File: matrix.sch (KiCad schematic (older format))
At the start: 143 parts

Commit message: Update: Work on PCB component placement
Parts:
- K_,1, K_.1, K_/1, K_;1, K_A1, K_B1, K_C1, K_D1, K_E1, K_F1, K_FN3, K_FN4_2, K_G1, K_H1, K_I1, K_J1, K_K1, K_L1, K_LALT1, K_M1, K_N1, K_O1, K_P1, K_Q1, K_R1, K_S1, K_T1, K_TAB1, K_U1, K_V1, K_W1, K_X1, K_Y1, K_Z1: footprint MX_Alps_Hybrid:MX-1U -> MX_Alps_Hybrid:MXOnly-1U
- K_BACK1, K_LSHIFT1: footprint MX_Alps_Hybrid:MX-1.75U -> MX_Alps_Hybrid:MXOnly-1.75U
- K_FN1: footprint MX_Alps_Hybrid:MX-1.25U -> MX_Alps_Hybrid:MXOnly-1.25U
- K_FN2: footprint MX_Alps_Hybrid:MX-1.5U -> MX_Alps_Hybrid:MXOnly-1.5U
- K_LCTL2, K_SUPER2: footprint MX_Alps_Hybrid:MX-1U -> MX_Alps_Hybrid:MXOnly-1U-FLIPPED

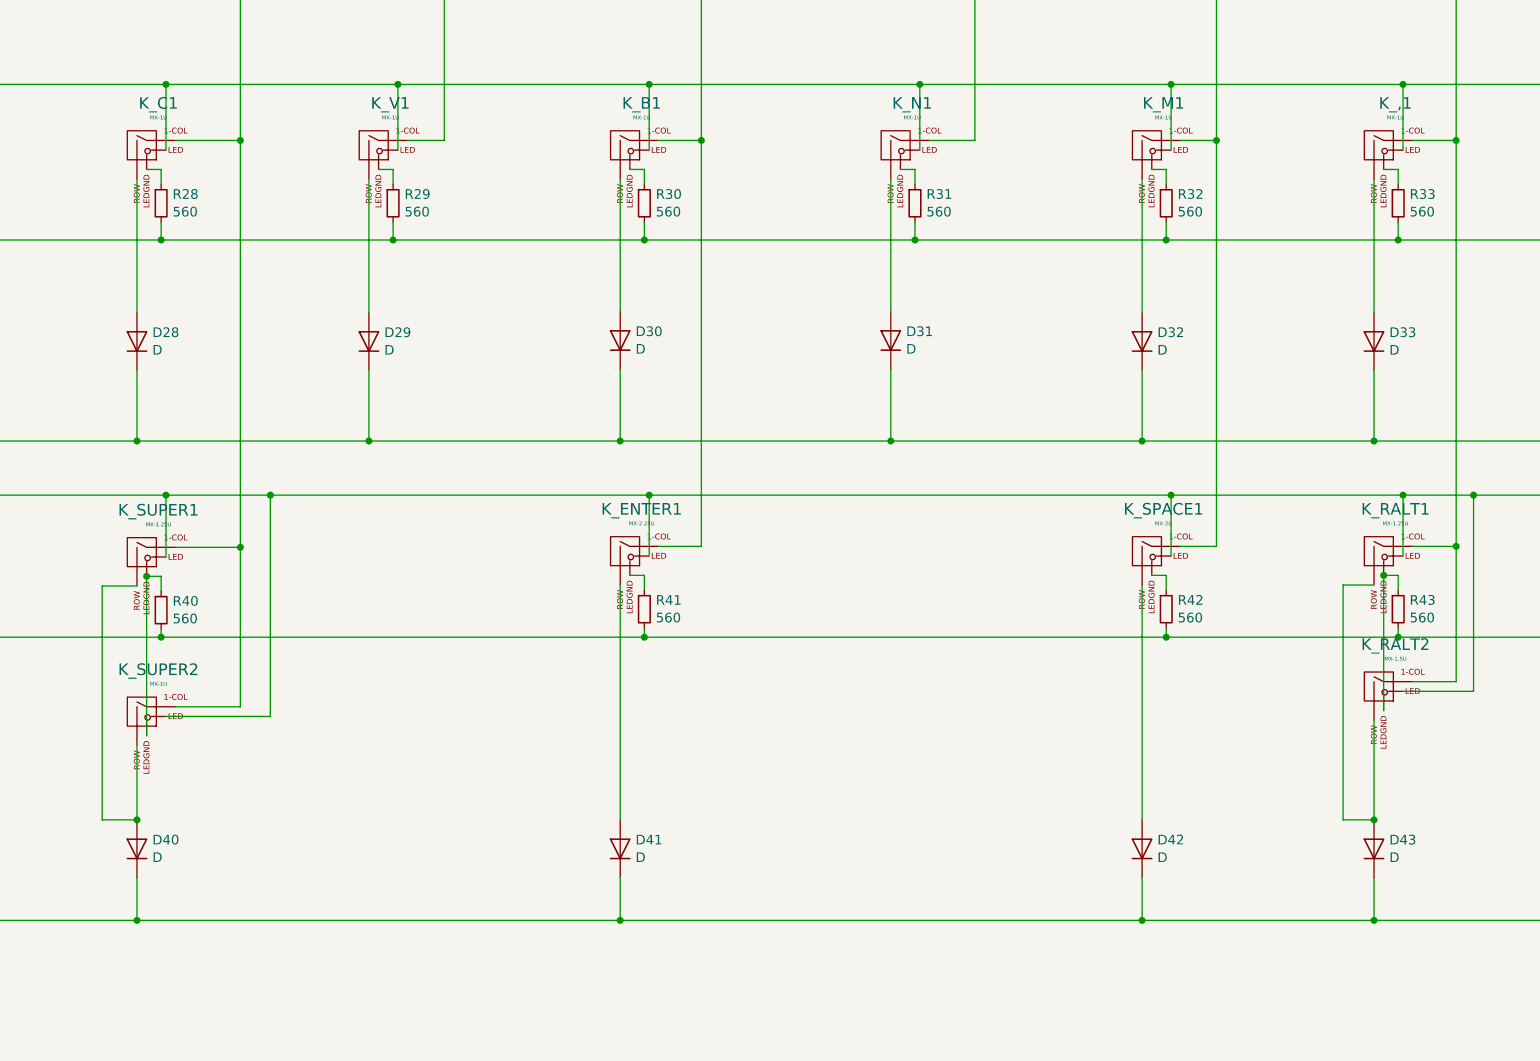
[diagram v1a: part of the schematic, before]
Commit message: Update: Work on PCB layout
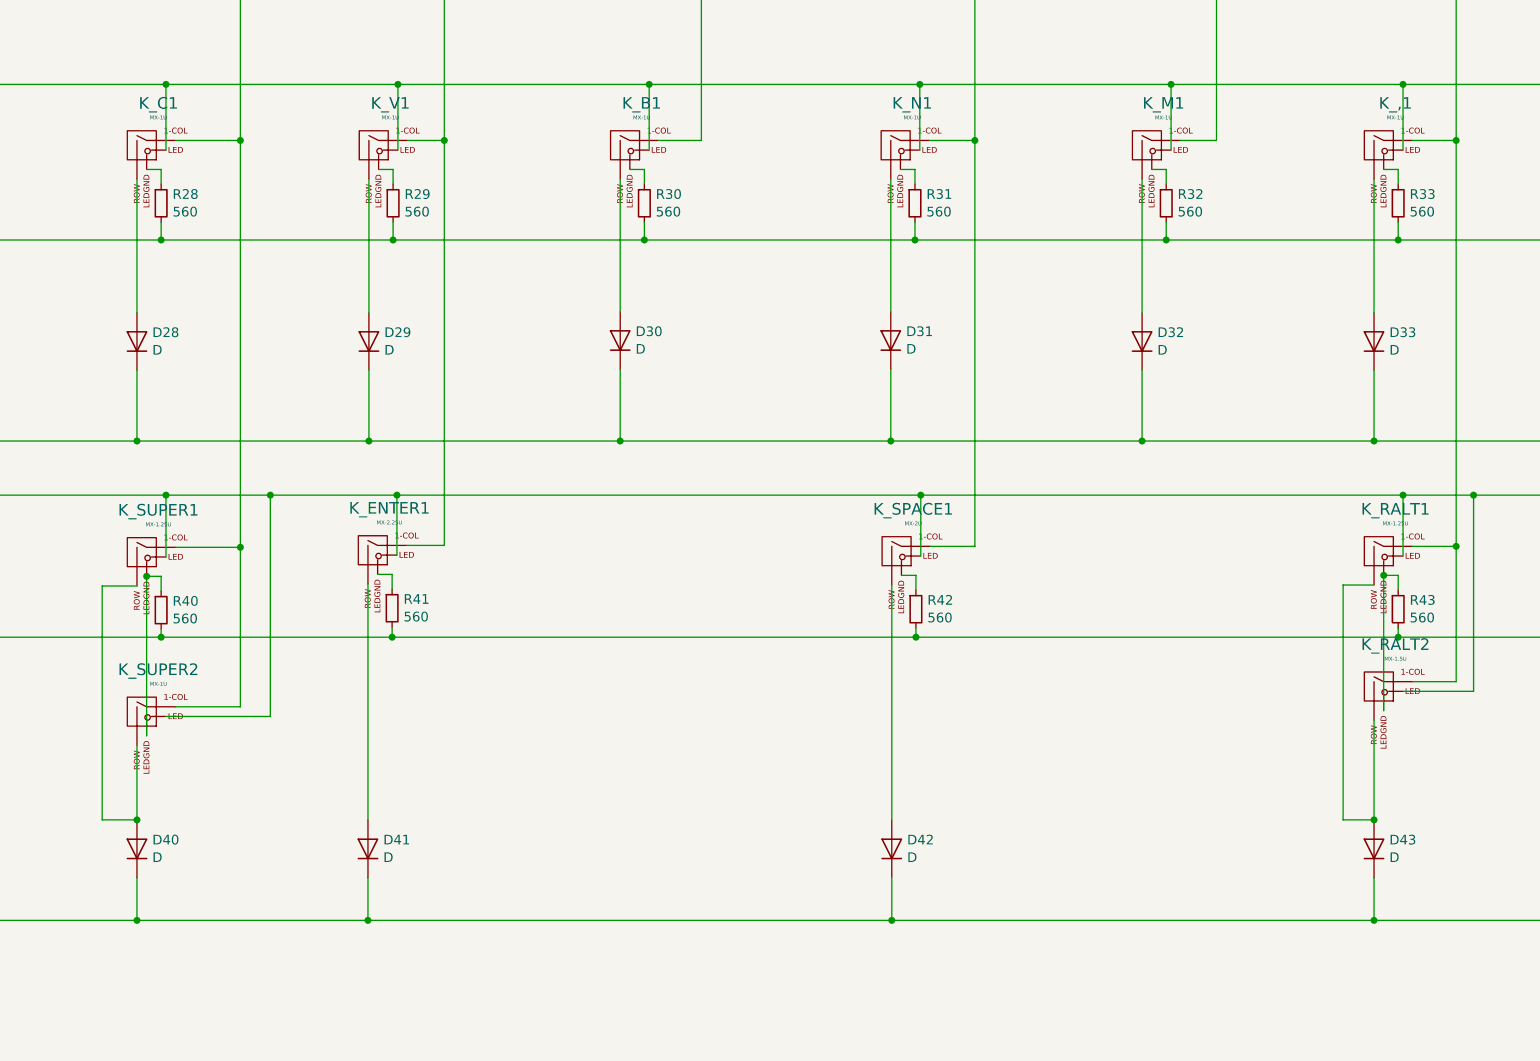
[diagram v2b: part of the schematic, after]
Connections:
- net COL4: now also K_ENTER1.1 (COL)
- net COL5: no longer K_ENTER1.1 (COL)
- net COL6: now also K_SPACE1.1 (COL)
- net COL7: no longer K_SPACE1.1 (COL)
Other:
- moved on the sheet: D41, D42, K_ENTER1, K_SPACE1, R41, R42
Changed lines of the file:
@@
 L MX_Alps_Hybrids:MX-2.25U K_ENTER1
 U 1 1 5C22137B
-P 7200 6800
-F 0 "K_ENTER1" H 7286 7017 60  0000 C CNN
-F 1 "MX-2.25U" H 7286 6943 20  0000 C CNN
-F 2 "MX_Alps_Hybrid:MXOnly-2.25U-ReversedStabilizers" H 7175 6775 60  0001 C CNN
-F 3 "" H 7175 6775 60  0001 C CNN
-	1    7200 6800
+P 5895 6795
+F 0 "K_ENTER1" H 5981 7012 60  0000 C CNN
+F 1 "MX-2.25U" H 5981 6938 20  0000 C CNN
+F 2 "MX_Alps_Hybrid:MXOnly-2.25U-ReversedStabilizers" H 5870 6770 60  0001 C CNN
+F 3 "" H 5870 6770 60  0001 C CNN
+	1    5895 6795
 	1    0    0    -1
 $EndComp
@@
 L MX_Alps_Hybrids:MX-2U K_SPACE1
 U 1 1 5C223C71
-P 9900 6800
-F 0 "K_SPACE1" H 9986 7017 60  0000 C CNN
-F 1 "MX-2U" H 9986 6943 20  0000 C CNN
-F 2 "MX_Alps_Hybrid:MXOnly-2U-ReversedStabilizers" H 9875 6775 60  0001 C CNN
-F 3 "" H 9875 6775 60  0001 C CNN
-	1    9900 6800
+P 8605 6800
+F 0 "K_SPACE1" H 8691 7017 60  0000 C CNN
+F 1 "MX-2U" H 8691 6943 20  0000 C CNN
+F 2 "MX_Alps_Hybrid:MXOnly-2U-ReversedStabilizers" H 8580 6775 60  0001 C CNN
+F 3 "" H 8580 6775 60  0001 C CNN
+	1    8605 6800
 	1    0    0    -1
 $EndComp
@@
 L Device:R_Small R41
 U 1 1 5C24348B
-P 7300 7100
-F 0 "R41" H 7359 7146 50  0000 L CNN
-F 1 "560" H 7359 7055 50  0000 L CNN
-F 2 "Resistor_SMD:R_0603_1608Metric" H 7300 7100 50  0001 C CNN
-F 3 "~" H 7300 7100 50  0001 C CNN
-	1    7300 7100
+P 5995 7095
+F 0 "R41" H 6054 7141 50  0000 L CNN
+F 1 "560" H 6054 7050 50  0000 L CNN
+F 2 "Resistor_SMD:R_0603_1608Metric" H 5995 7095 50  0001 C CNN
+F 3 "~" H 5995 7095 50  0001 C CNN
+	1    5995 7095
 	1    0    0    -1
 $EndComp
@@
 L Device:R_Small R42
 U 1 1 5C2440AF
-P 10000 7100
-F 0 "R42" H 10059 7146 50  0000 L CNN
-F 1 "560" H 10059 7055 50  0000 L CNN
-F 2 "Resistor_SMD:R_0603_1608Metric" H 10000 7100 50  0001 C CNN
-F 3 "~" H 10000 7100 50  0001 C CNN
-	1    10000 7100
+P 8705 7100
+F 0 "R42" H 8764 7146 50  0000 L CNN
+F 1 "560" H 8764 7055 50  0000 L CNN
+F 2 "Resistor_SMD:R_0603_1608Metric" H 8705 7100 50  0001 C CNN
+F 3 "~" H 8705 7100 50  0001 C CNN
+	1    8705 7100
 	1    0    0    -1
 $EndComp
@@
 	4800 6930 4800 7005
 Wire Wire Line
-	7225 6925 7300 6925
-Wire Wire Line
-	7300 6925 7300 7000
-Wire Wire Line
-	9925 6925 10000 6925
-Wire Wire Line
-	10000 6925 10000 7000
+	5920 6920 5995 6920
+Wire Wire Line
+	5995 6920 5995 6995
+Wire Wire Line
+	8630 6925 8705 6925
+Wire Wire Line
+	8705 6925 8705 7000
 Wire Wire Line
 	11125 6925 11200 6925
@@
 Connection ~ 2300 7245
 Wire Wire Line
-	7300 7200 7300 7245
-Wire Wire Line
-	10000 7200 10000 7245
-Wire Wire Line
-	10000 7245 7300 7245
-Connection ~ 7300 7245
-Wire Wire Line
 	11200 7200 11200 7245
-Wire Wire Line
-	11200 7245 10000 7245
-Connection ~ 10000 7245
 Wire Wire Line
 	12500 7200 12500 7245
@@
 	11225 6510 11225 6825
 Connection ~ 12525 6510
-Wire Wire Line
-	10025 6510 10025 6825
 Connection ~ 11225 6510
-Wire Wire Line
-	7325 6510 7325 6825
-Connection ~ 10025 6510
-Connection ~ 7325 6510
 Wire Wire Line
 	2325 6510 2325 6825
@@
 COL5
 Wire Wire Line
-	7375 6775 7595 6775
-Wire Wire Line
 	7595 750  7595 1275
 Wire Wire Line
 	7375 4675 7595 4675
-Connection ~ 7595 4675
-Wire Wire Line
-	7595 4675 7595 6775
 Wire Wire Line
 	7375 2675 7595 2675
@@
 	10260 750  10260 1275
 Wire Wire Line
-	10075 6775 10260 6775
-Wire Wire Line
 	10075 4675 10260 4675
-Connection ~ 10260 4675
-Wire Wire Line
-	10260 4675 10260 6775
 Wire Wire Line
 	10075 2675 10260 2675
@@
 Wire Wire Line
 	12525 6510 13725 6510
-Wire Wire Line
-	7325 6510 10025 6510
-Wire Wire Line
-	10025 6510 11225 6510
 Wire Wire Line
 	865  2200 975  2200
@@
 	4800 7205 4800 7245
 Connection ~ 4800 7245
-Wire Wire Line
-	4800 7245 7300 7245
 $Comp
 L MX_Alps_Hybrids:MX-1U K_LCTL2
@@
 Connection ~ 4675 8710
 Wire Wire Line
-	4675 8710 7175 8710
-Wire Wire Line
 	1025 7760 1025 6925
 Connection ~ 1025 6925
@@
 L Device:D D41
 U 1 1 5E87BBD0
-P 7175 8340
-F 0 "D41" V 7221 8261 50  0000 R CNN
-F 1 "D" V 7130 8261 50  0000 R CNN
-F 2 "Diode_SMD:D_SOD-123" H 7175 8340 50  0001 C CNN
-F 3 "http://www.mccsemi.com/up_pdf/1N4148W(SOD123).pdf" H 7175 8340 50  0001 C CNN
-F 4 "C83528" V 7175 8340 50  0001 C CNN "LCSC PN"
-F 5 "1N4148W-TP" V 7175 8340 50  0001 C CNN "Product"
-	1    7175 8340
-	0    -1   -1   0
-$EndComp
-Wire Wire Line
-	7175 6975 7175 8190
-Wire Wire Line
-	7175 8490 7175 8710
-Connection ~ 7175 8710
-Wire Wire Line
-	7175 8710 9875 8710
+P 5870 8340
+F 0 "D41" V 5916 8261 50  0000 R CNN
+F 1 "D" V 5825 8261 50  0000 R CNN
+F 2 "Diode_SMD:D_SOD-123" H 5870 8340 50  0001 C CNN
+F 3 "http://www.mccsemi.com/up_pdf/1N4148W(SOD123).pdf" H 5870 8340 50  0001 C CNN
+F 4 "C83528" V 5870 8340 50  0001 C CNN "LCSC PN"
+F 5 "1N4148W-TP" V 5870 8340 50  0001 C CNN "Product"
+	1    5870 8340
+	0    -1   -1   0
+$EndComp
 $Comp
 L Device:D D42
 U 1 1 5E9157F4
-P 9875 8340
-F 0 "D42" V 9921 8261 50  0000 R CNN
-F 1 "D" V 9830 8261 50  0000 R CNN
-F 2 "Diode_SMD:D_SOD-123" H 9875 8340 50  0001 C CNN
-F 3 "http://www.mccsemi.com/up_pdf/1N4148W(SOD123).pdf" H 9875 8340 50  0001 C CNN
-F 4 "C83528" V 9875 8340 50  0001 C CNN "LCSC PN"
-F 5 "1N4148W-TP" V 9875 8340 50  0001 C CNN "Product"
-	1    9875 8340
-	0    -1   -1   0
-$EndComp
-Wire Wire Line
-	9875 6975 9875 8190
-Wire Wire Line
-	9875 8490 9875 8710
-Connection ~ 9875 8710
-Wire Wire Line
-	9875 8710 11075 8710
+P 8580 8340
+F 0 "D42" V 8626 8261 50  0000 R CNN
+F 1 "D" V 8535 8261 50  0000 R CNN
+F 2 "Diode_SMD:D_SOD-123" H 8580 8340 50  0001 C CNN
+F 3 "http://www.mccsemi.com/up_pdf/1N4148W(SOD123).pdf" H 8580 8340 50  0001 C CNN
+F 4 "C83528" V 8580 8340 50  0001 C CNN "LCSC PN"
+F 5 "1N4148W-TP" V 8580 8340 50  0001 C CNN "Product"
+	1    8580 8340
+	0    -1   -1   0
+$EndComp
 $Comp
 L Device:D D43
@@
 Connection ~ 5365 6510
 Wire Wire Line
-	5365 6510 7325 6510
+	5365 6510 6020 6510
+Wire Wire Line
+	4675 8710 5870 8710
+Wire Wire Line
+	4800 7245 5995 7245
+Wire Wire Line
+	5870 8490 5870 8710
+Connection ~ 5870 8710
+Wire Wire Line
+	5870 6970 5870 8190
+Wire Wire Line
+	5995 7195 5995 7245
+Connection ~ 5995 7245
+Wire Wire Line
+	6070 6770 6265 6770
+Wire Wire Line
+	6265 6770 6265 4675
+Connection ~ 6265 4675
+Wire Wire Line
+	6020 6820 6020 6510
+Connection ~ 6020 6510
+Wire Wire Line
+	5870 8710 8580 8710
+Wire Wire Line
+	5995 7245 8705 7245
+Wire Wire Line
+	6020 6510 8730 6510
+Wire Wire Line
+	8705 7200 8705 7245
+Connection ~ 8705 7245
+Wire Wire Line
+	8705 7245 11200 7245
+Wire Wire Line
+	8730 6825 8730 6510
+Connection ~ 8730 6510
+Wire Wire Line
+	8730 6510 11225 6510
+Wire Wire Line
+	8780 6775 9010 6775
+Wire Wire Line
+	9010 6775 9010 4675
+Connection ~ 9010 4675
+Wire Wire Line
+	8580 6975 8580 8190
+Wire Wire Line
+	8580 8490 8580 8710
+Connection ~ 8580 8710
+Wire Wire Line
+	8580 8710 11075 8710
 $EndSCHEMATC
